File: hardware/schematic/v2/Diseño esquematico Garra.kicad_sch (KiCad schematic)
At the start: 15 parts

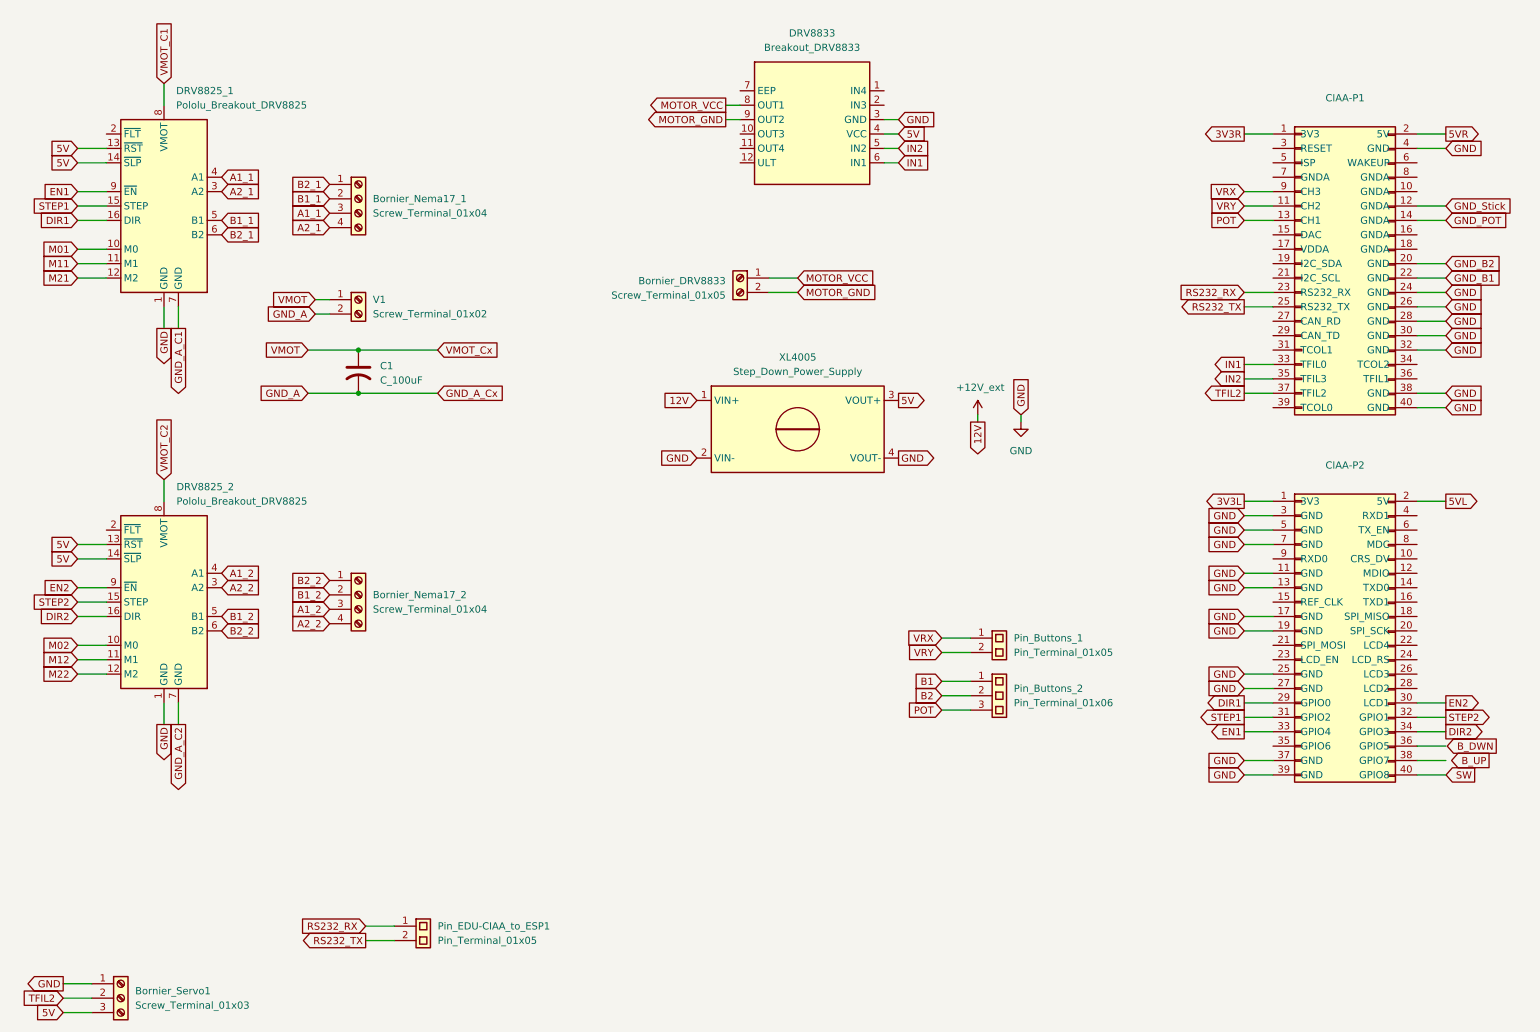
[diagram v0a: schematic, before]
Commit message: PCB Updated
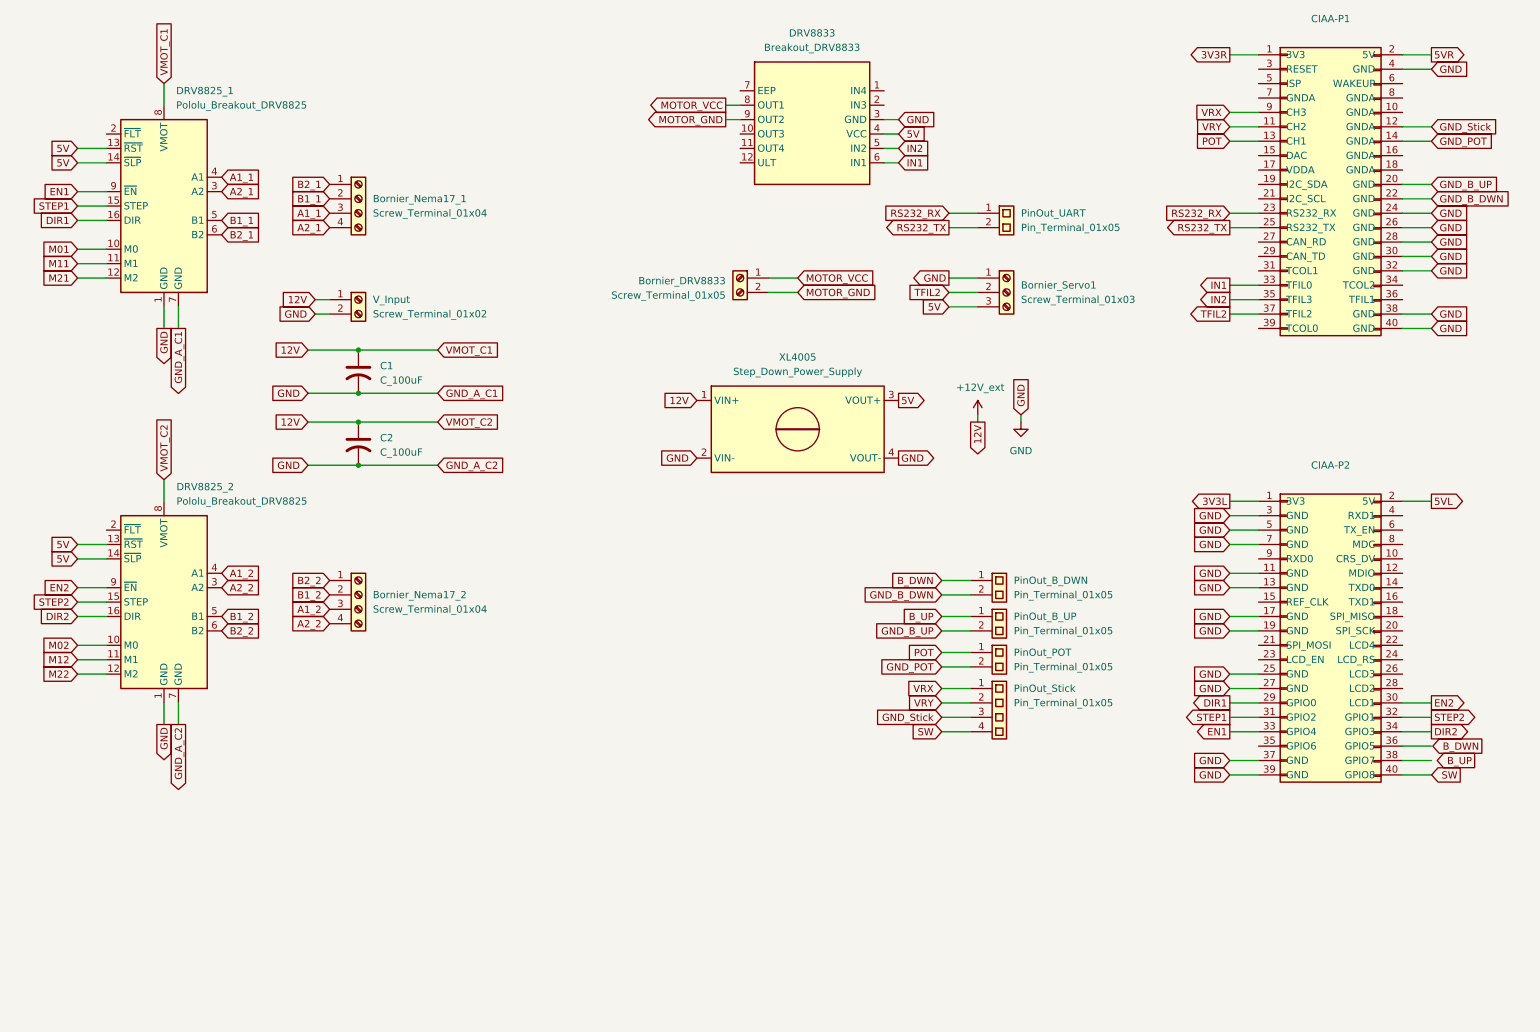
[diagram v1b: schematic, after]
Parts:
- removed Pin_Buttons_2: Pin_Terminal_01x06, Connector_PinSocket_2.00mm:PinSocket_1x03_P2.00mm_Vertical, symbol Connector:Screw_Terminal_01x03
- added C2: C_100uF, Capacitor_THT:C_Radial_D8.0mm_H11.5mm_P3.50mm, symbol Device:C_US
- added PinOut_B_DWN, PinOut_B_UP, PinOut_POT: Pin_Terminal_01x05, Connector_PinSocket_2.00mm:PinSocket_1x02_P2.00mm_Vertical, symbol Connector:Screw_Terminal_01x02
- CIAA-P1, CIAA-P2: footprint Connector_PinHeader_1.00mm:PinHeader_1x20_P1.00mm_Vertical -> Libreria_EDU_CIAA_NXP:PIN_ARRAY_20X2
- PinOut_Stick: renamed from Pin_Buttons_1; footprint Connector_PinSocket_2.00mm:PinSocket_1x02_P2.00mm_Vertical -> Connector_PinSocket_2.00mm:PinSocket_1x04_P2.00mm_Vertical
- renumbered Pin_EDU-CIAA_to_ESP1 to PinOut_UART, V1 to V_Input
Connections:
- net GND_A is gone; now on net GND: C1.2, V_Input.2 (Pin_2)
- net GND_A_C1 is gone; now on net GND: DRV8825_1.7 (GND)
- net GND_A_C2 is gone; now on net GND: DRV8825_2.7 (GND)
- net VMOT is gone; now on net +12V_ext: C1.1, V_Input.1 (Pin_1)
- net VMOT_C1 is gone; now on net +12V_ext: DRV8825_1.8 (VMOT)
- net VMOT_C2 is gone; now on net +12V_ext: DRV8825_2.8 (VMOT)
- net +12V_ext: now also C2.1
- net B_DWN: now also PinOut_B_DWN.1 (Pin_1)
- net B_UP: now also PinOut_B_UP.1 (Pin_1)
- net GND: now also C2.2
- net GND_POT: now also PinOut_POT.2 (Pin_2)
- net GND_Stick: now also PinOut_Stick.3 (Pin_3)
- net POT: now also PinOut_POT.1 (Pin_1)
- net SW: now also PinOut_Stick.4 (Pin_4)
- net GND_B1 renamed GND_B_DWN
- net GND_B_DWN: now also PinOut_B_DWN.2 (Pin_2)
- net GND_B2 renamed GND_B_UP
- net GND_B_UP: now also PinOut_B_UP.2 (Pin_2)
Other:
- moved on the sheet: Bornier_Servo1, CIAA-P1, CIAA-P2, PinOut_UART
